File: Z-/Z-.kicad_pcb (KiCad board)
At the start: 4 copper layers, 98 x 98 mm, 144 parts, among them J1 200528-0100, J2 U.FL, J3 U.FL, J4 200528-0100, J5 Conn_01x02, K1 IM02DGR, Q1 NX3008NBKS, Q10 NX3008NBKS, Q11 IRLML2803, Q12 MBT2222ADW1T1, Q13 IRLML2803, Q14 NX3008NBKS, Q15 IRF7404, Q16 MBT2222ADW1T1, Q17 IRF7404, Q18 IRLML2803, Q19 IRF7404, Q2 NX3008NBKS, Q3 MBT2222ADW1T1, Q4 MBT2222ADW1T1, Q5 NX3008NBKS, Q6 NX3008NBKS, Q7 MBT2222ADW1T1, Q8 MBT2222ADW1T1, Q9 MMBT2222AT, U1 OPT4003DNPRQ1, U2 LTC4316xDD, U3 ADM1176-1ARMZ-R7, U4 NCV891330PD50R2G, U5 DRV8830DRC

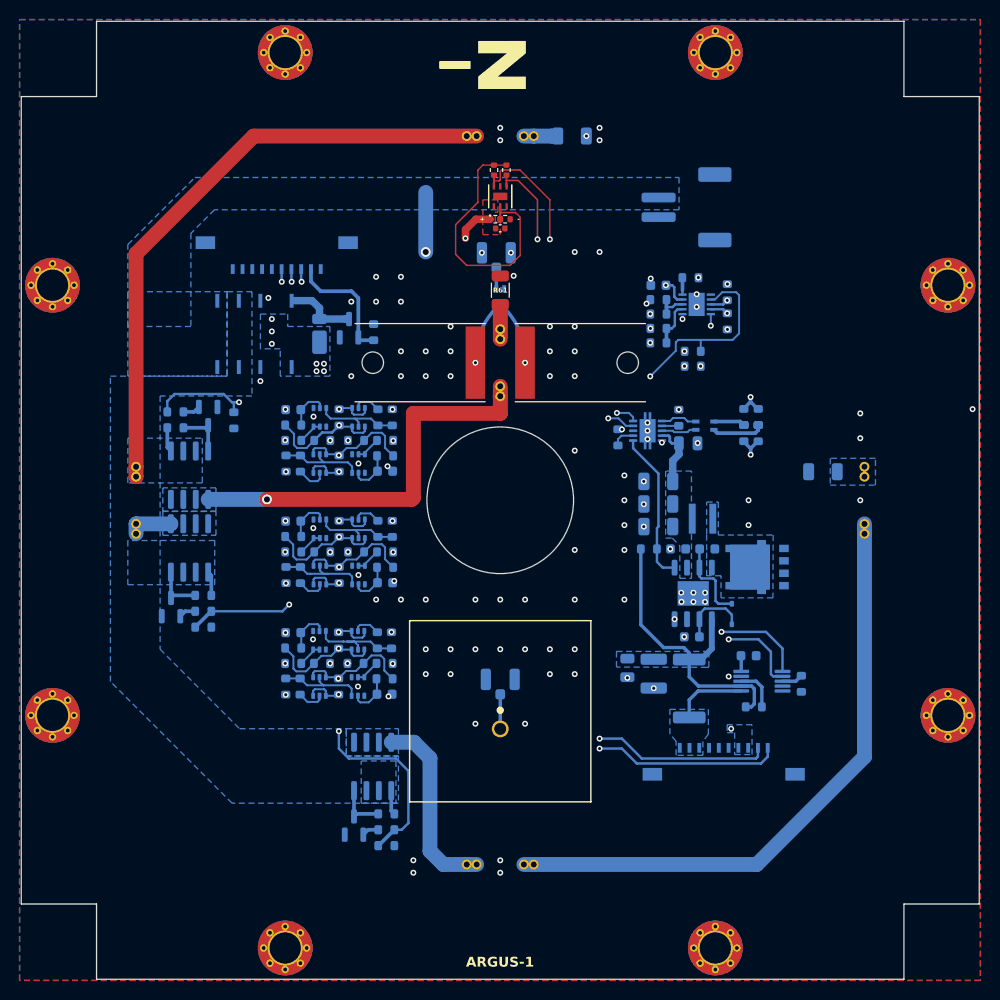
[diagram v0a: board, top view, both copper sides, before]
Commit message: Z- Solar Panel files upload
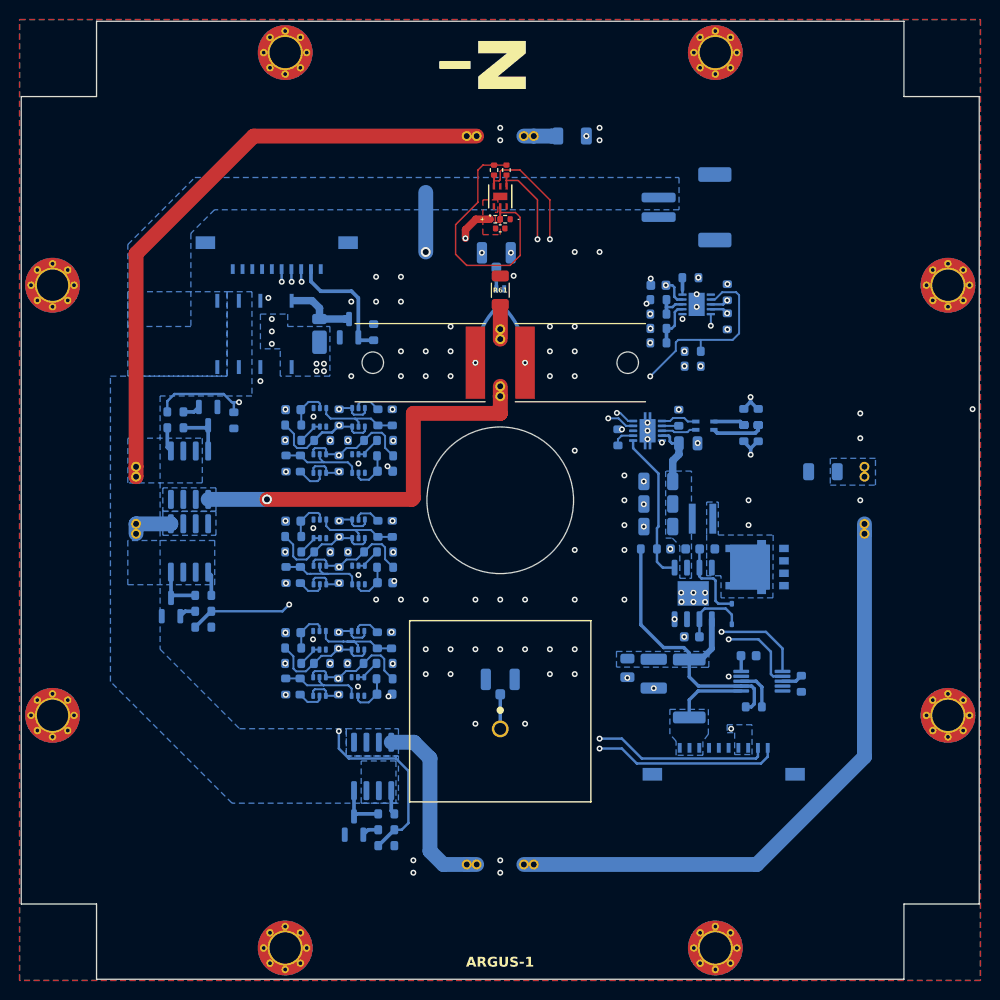
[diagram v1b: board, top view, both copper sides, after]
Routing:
- net VDRIVE: track 32.0 -> 30.6 mm
- net SDA: track 97.2 -> 96.6 mm
- net SCL: track 90.8 -> 90.2 mm
- net Net-(D1-A): track 7.13 -> 6.58 mm
